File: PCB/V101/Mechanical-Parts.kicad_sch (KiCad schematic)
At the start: 4 parts

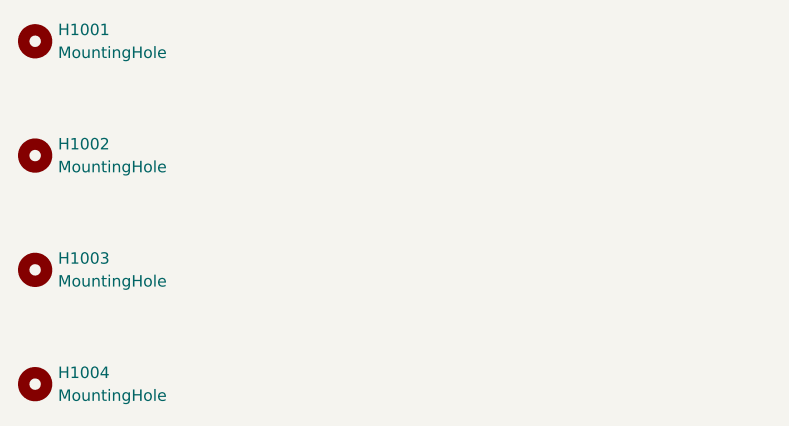
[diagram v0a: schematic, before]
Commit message: Updated PCB
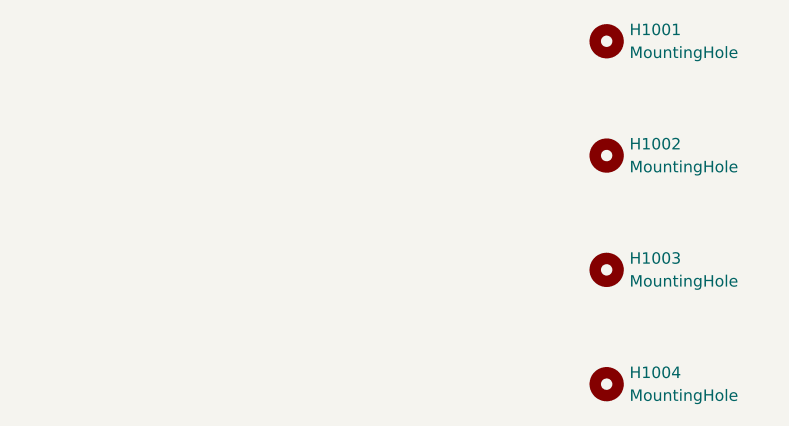
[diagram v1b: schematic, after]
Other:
- moved on the sheet: H1001, H1002, H1003, H1004
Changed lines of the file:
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@@
 	(symbol
 		(lib_id "Mechanical:MountingHole")
-		(at 88.9 101.6 0)
+		(at 152.4 101.6 0)
 		(unit 1)
 		(exclude_from_sim no)
@@
 		(fields_autoplaced yes)
 		(property "Reference" "H1003"
-			(at 91.44 100.3299 0)
-			(effects
-				(font
-					(size 1.27 1.27)
-				)
-				(justify left)
-			)
-		)
-		(property "Value" "MountingHole"
-			(at 91.44 102.8699 0)
-			(effects
-				(font
-					(size 1.27 1.27)
-				)
-				(justify left)
-			)
-		)
-		(property "Footprint" "MountingHole:MountingHole_3.2mm_M3"
-			(at 88.9 101.6 0)
-			(effects
-				(font
-					(size 1.27 1.27)
-				)
-				(hide yes)
-			)
-		)
-		(property "Datasheet" "~"
-			(at 88.9 101.6 0)
-			(effects
-				(font
-					(size 1.27 1.27)
-				)
-				(hide yes)
-			)
-		)
-		(property "Description" "Mounting Hole without connection"
-			(at 88.9 101.6 0)
+			(at 154.94 100.3299 0)
+			(effects
+				(font
+					(size 1.27 1.27)
+				)
+				(justify left)
+			)
+		)
+		(property "Value" "MountingHole"
+			(at 154.94 102.8699 0)
+			(effects
+				(font
+					(size 1.27 1.27)
+				)
+				(justify left)
+			)
+		)
+		(property "Footprint" "MountingHole:MountingHole_3.2mm_M3"
+			(at 152.4 101.6 0)
+			(effects
+				(font
+					(size 1.27 1.27)
+				)
+				(hide yes)
+			)
+		)
+		(property "Datasheet" "~"
+			(at 152.4 101.6 0)
+			(effects
+				(font
+					(size 1.27 1.27)
+				)
+				(hide yes)
+			)
+		)
+		(property "Description" "Mounting Hole without connection"
+			(at 152.4 101.6 0)
 			(effects
 				(font
@@
 	(symbol
 		(lib_id "Mechanical:MountingHole")
-		(at 88.9 114.3 0)
+		(at 152.4 114.3 0)
 		(unit 1)
 		(exclude_from_sim no)
@@
 		(fields_autoplaced yes)
 		(property "Reference" "H1004"
-			(at 91.44 113.0299 0)
-			(effects
-				(font
-					(size 1.27 1.27)
-				)
-				(justify left)
-			)
-		)
-		(property "Value" "MountingHole"
-			(at 91.44 115.5699 0)
-			(effects
-				(font
-					(size 1.27 1.27)
-				)
-				(justify left)
-			)
-		)
-		(property "Footprint" "MountingHole:MountingHole_3.2mm_M3"
-			(at 88.9 114.3 0)
-			(effects
-				(font
-					(size 1.27 1.27)
-				)
-				(hide yes)
-			)
-		)
-		(property "Datasheet" "~"
-			(at 88.9 114.3 0)
-			(effects
-				(font
-					(size 1.27 1.27)
-				)
-				(hide yes)
-			)
-		)
-		(property "Description" "Mounting Hole without connection"
-			(at 88.9 114.3 0)
+			(at 154.94 113.0299 0)
+			(effects
+				(font
+					(size 1.27 1.27)
+				)
+				(justify left)
+			)
+		)
+		(property "Value" "MountingHole"
+			(at 154.94 115.5699 0)
+			(effects
+				(font
+					(size 1.27 1.27)
+				)
+				(justify left)
+			)
+		)
+		(property "Footprint" "MountingHole:MountingHole_3.2mm_M3"
+			(at 152.4 114.3 0)
+			(effects
+				(font
+					(size 1.27 1.27)
+				)
+				(hide yes)
+			)
+		)
+		(property "Datasheet" "~"
+			(at 152.4 114.3 0)
+			(effects
+				(font
+					(size 1.27 1.27)
+				)
+				(hide yes)
+			)
+		)
+		(property "Description" "Mounting Hole without connection"
+			(at 152.4 114.3 0)
 			(effects
 				(font
@@
 	(symbol
 		(lib_id "Mechanical:MountingHole")
-		(at 88.9 88.9 0)
+		(at 152.4 88.9 0)
 		(unit 1)
 		(exclude_from_sim no)
@@
 		(fields_autoplaced yes)
 		(property "Reference" "H1002"
-			(at 91.44 87.6299 0)
-			(effects
-				(font
-					(size 1.27 1.27)
-				)
-				(justify left)
-			)
-		)
-		(property "Value" "MountingHole"
-			(at 91.44 90.1699 0)
-			(effects
-				(font
-					(size 1.27 1.27)
-				)
-				(justify left)
-			)
-		)
-		(property "Footprint" "MountingHole:MountingHole_3.2mm_M3"
-			(at 88.9 88.9 0)
-			(effects
-				(font
-					(size 1.27 1.27)
-				)
-				(hide yes)
-			)
-		)
-		(property "Datasheet" "~"
-			(at 88.9 88.9 0)
-			(effects
-				(font
-					(size 1.27 1.27)
-				)
-				(hide yes)
-			)
-		)
-		(property "Description" "Mounting Hole without connection"
-			(at 88.9 88.9 0)
+			(at 154.94 87.6299 0)
+			(effects
+				(font
+					(size 1.27 1.27)
+				)
+				(justify left)
+			)
+		)
+		(property "Value" "MountingHole"
+			(at 154.94 90.1699 0)
+			(effects
+				(font
+					(size 1.27 1.27)
+				)
+				(justify left)
+			)
+		)
+		(property "Footprint" "MountingHole:MountingHole_3.2mm_M3"
+			(at 152.4 88.9 0)
+			(effects
+				(font
+					(size 1.27 1.27)
+				)
+				(hide yes)
+			)
+		)
+		(property "Datasheet" "~"
+			(at 152.4 88.9 0)
+			(effects
+				(font
+					(size 1.27 1.27)
+				)
+				(hide yes)
+			)
+		)
+		(property "Description" "Mounting Hole without connection"
+			(at 152.4 88.9 0)
 			(effects
 				(font
@@
 	(symbol
 		(lib_id "Mechanical:MountingHole")
-		(at 88.9 76.2 0)
+		(at 152.4 76.2 0)
 		(unit 1)
 		(exclude_from_sim no)
@@
 		(fields_autoplaced yes)
 		(property "Reference" "H1001"
-			(at 91.44 74.9299 0)
-			(effects
-				(font
-					(size 1.27 1.27)
-				)
-				(justify left)
-			)
-		)
-		(property "Value" "MountingHole"
-			(at 91.44 77.4699 0)
-			(effects
-				(font
-					(size 1.27 1.27)
-				)
-				(justify left)
-			)
-		)
-		(property "Footprint" "MountingHole:MountingHole_3.2mm_M3"
-			(at 88.9 76.2 0)
-			(effects
-				(font
-					(size 1.27 1.27)
-				)
-				(hide yes)
-			)
-		)
-		(property "Datasheet" "~"
-			(at 88.9 76.2 0)
-			(effects
-				(font
-					(size 1.27 1.27)
-				)
-				(hide yes)
-			)
-		)
-		(property "Description" "Mounting Hole without connection"
-			(at 88.9 76.2 0)
-			(effects
-				(font
+			(at 154.94 74.9299 0)
+			(effects
+				(font
+					(size 1.27 1.27)
+				)
+				(justify left)
+			)
+		)
+		(property "Value" "MountingHole"
+			(at 154.94 77.4699 0)
+			(effects
+				(font
+					(size 1.27 1.27)
+				)
+				(justify left)
+			)
+		)
+		(property "Footprint" "MountingHole:MountingHole_3.2mm_M3"
+			(at 152.4 76.2 0)
+			(effects
+				(font
+					(size 1.27 1.27)
+				)
+				(hide yes)
+			)
+		)
+		(property "Datasheet" "~"
+			(at 152.4 76.2 0)
+			(effects
+				(font
+					(size 1.27 1.27)
+				)
+				(hide yes)
+			)
+		)
+		(property "Description" "Mounting Hole without connection"
+			(at 152.4 76.2 0)
+			(effects
+				(font
